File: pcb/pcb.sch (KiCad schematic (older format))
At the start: 44 parts, among them J1 USB_B_Mini, J4 UART_BUS, Q1 BSS138DW-7-F, SW1 PTS645Vx83, SW2 PTS645Vx83, SW3 PTS645Vx83, SW4 KMR2, U1 AP2112K-3.3, U2 MIC5225-1.8YM5, U3 CP2104, U5 ESP-12F

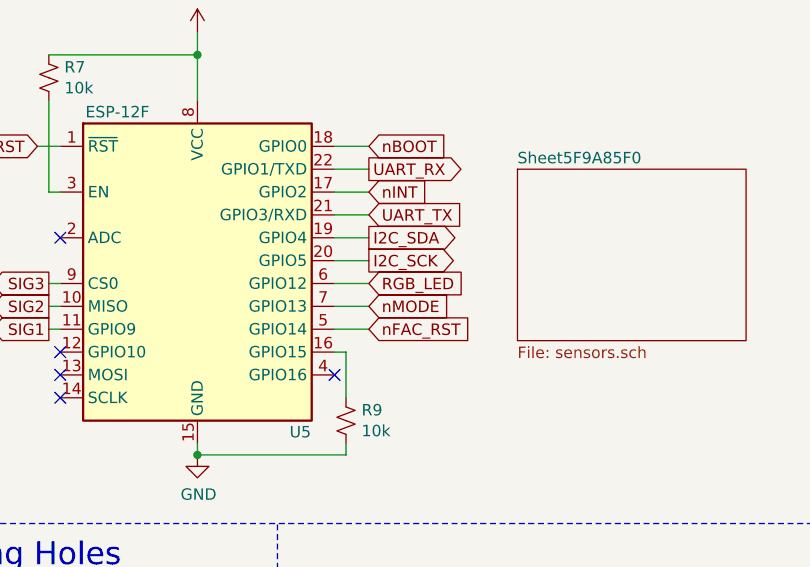
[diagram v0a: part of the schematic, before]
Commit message: cleaning up logic
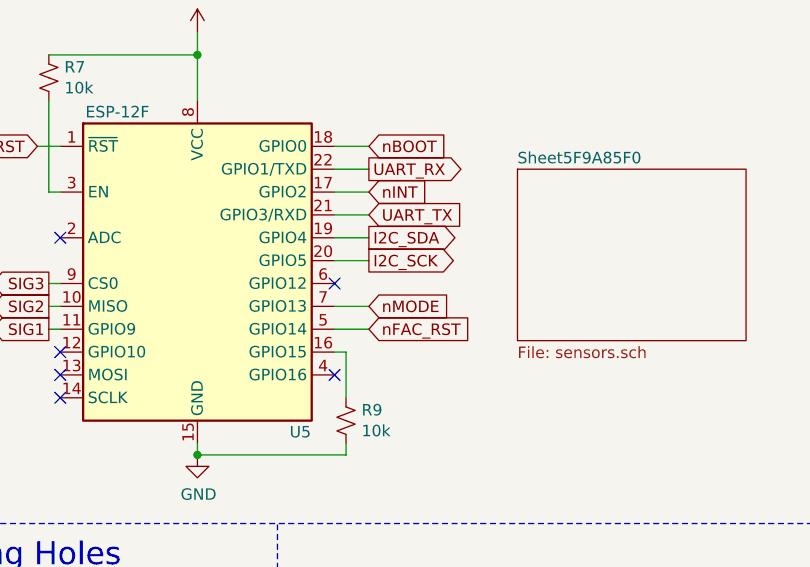
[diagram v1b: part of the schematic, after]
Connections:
- net RGB_LED: no longer names the net of U5.6 (GPIO12)
- no-connect marks 20 -> 21
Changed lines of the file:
@@
 Wire Wire Line
 	3500 3650 4350 3650
-Text GLabel 7850 2100 2    50   Input ~ 0
-RGB_LED
-Wire Wire Line
-	7700 2100 7850 2100
 Wire Wire Line
 	7700 1700 7850 1700
@@
 F 3 "~" H 4300 1700 50  0001 C CNN
 	1    4300 1700
-	1    0    0    -1
-$EndComp
-$Comp
-L Regulator_Linear:AP2112K-3.3 U1
-U 1 1 5F256A82
-P 3850 1500
-F 0 "U1" H 3850 1842 50  0000 C CNN
-F 1 "AP2112K-3.3" H 3850 1751 50  0000 C CNN
-F 2 "Package_TO_SOT_SMD:SOT-23-5" H 3850 1825 50  0001 C CNN
-F 3 "https://www.diodes.com/assets/Datasheets/AP2112.pdf" H 3850 1600 50  0001 C CNN
-	1    3850 1500
 	1    0    0    -1
 $EndComp
@@
 Wire Wire Line
 	6450 2300 6500 2300
+$Comp
+L Regulator_Linear:AP2112K-3.3 U1
+U 1 1 5F256A82
+P 3850 1500
+F 0 "U1" H 3850 1842 50  0000 C CNN
+F 1 "AP2112K-3.3" H 3850 1751 50  0000 C CNN
+F 2 "Package_TO_SOT_SMD:SOT-23-5" H 3850 1825 50  0001 C CNN
+F 3 "https://www.diodes.com/assets/Datasheets/AP2112.pdf" H 3850 1600 50  0001 C CNN
+	1    3850 1500
+	1    0    0    -1
+$EndComp
+NoConn ~ 7700 2100
 $EndSCHEMATC
